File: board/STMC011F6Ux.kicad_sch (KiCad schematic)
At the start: 10 parts, among them J5 STDC14, SW1 SW_Push, U1 STM32C011F6Ux, Y1 48MHz

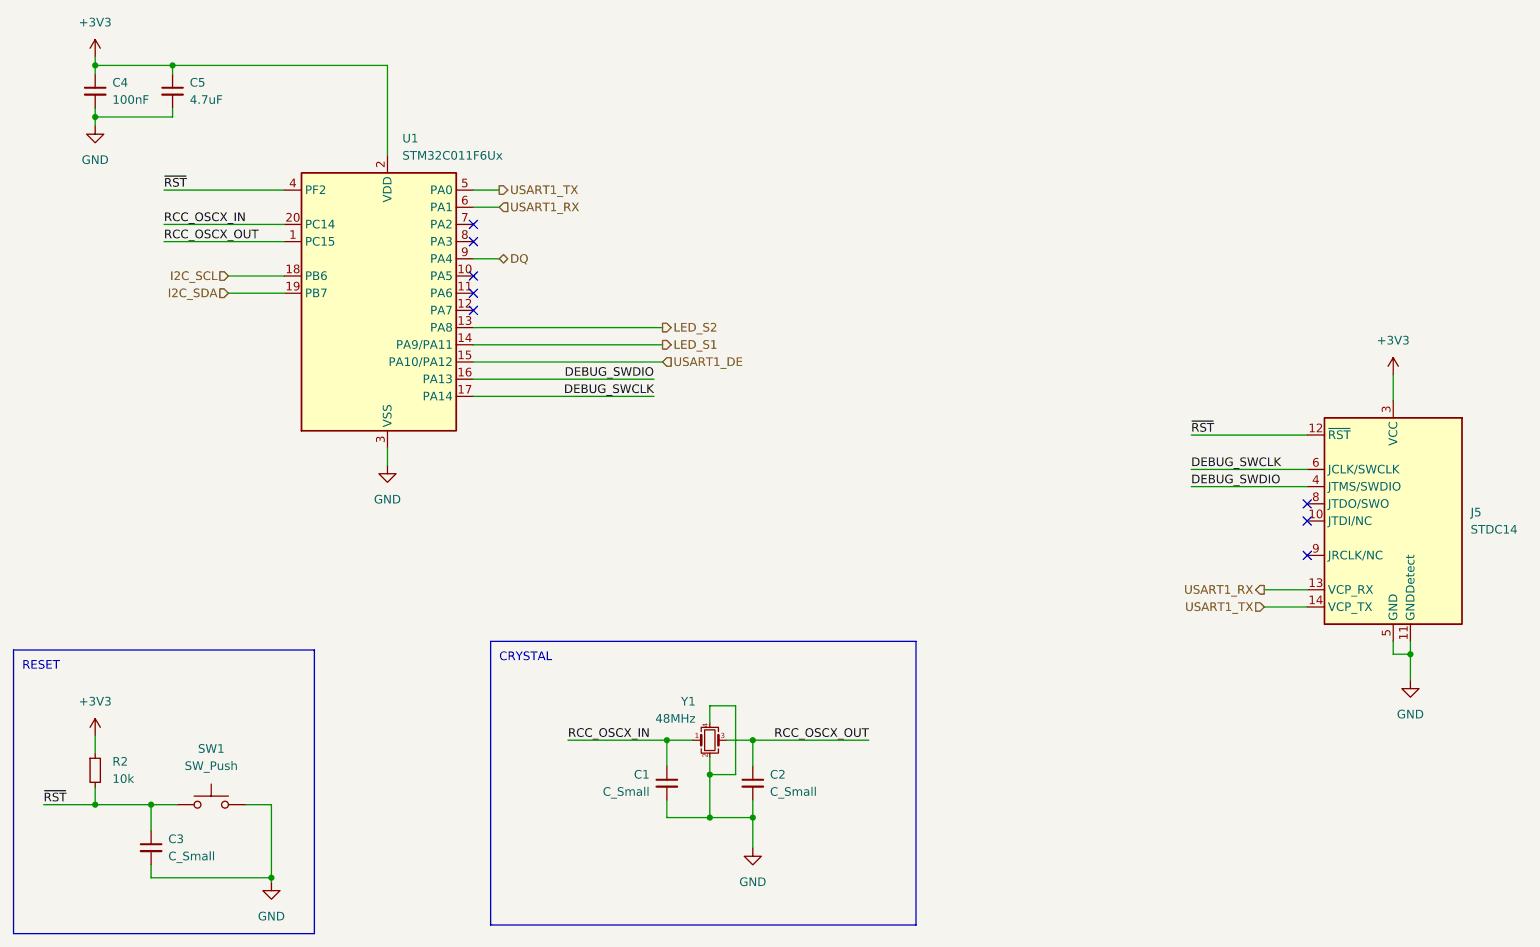
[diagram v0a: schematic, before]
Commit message: Final update
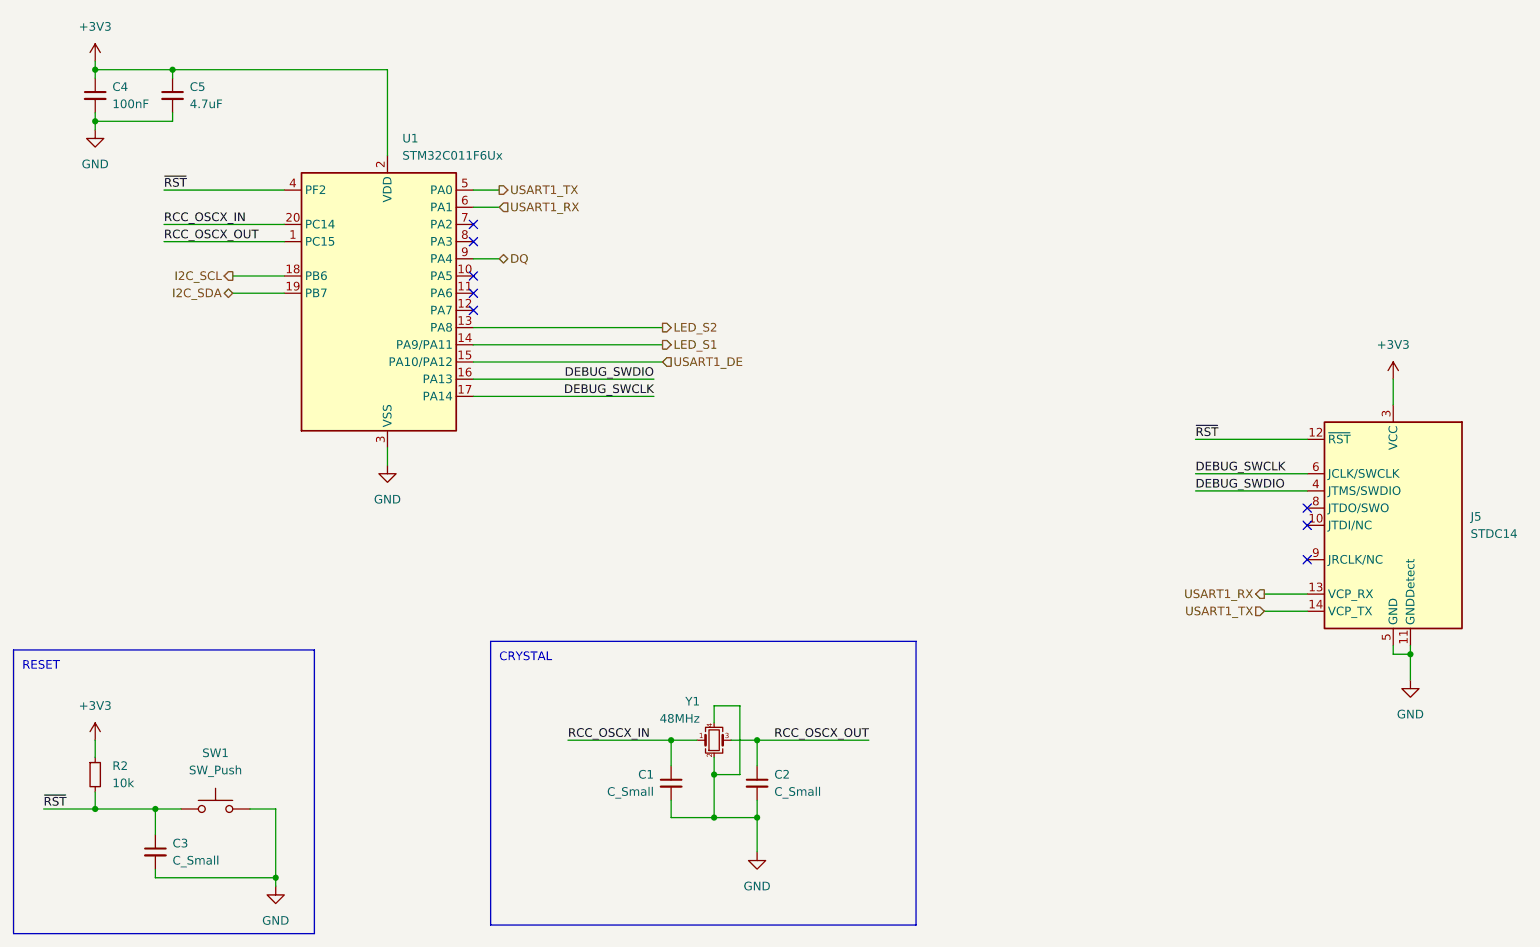
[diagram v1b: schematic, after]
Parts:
- SW1: footprint Connector_PinHeader_2.54mm:PinHeader_1x02_P2.54mm_Vertical -> Aliexpress:Push_Button_G71Y_3X6X3.5MM
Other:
- moved on the sheet: C1, C2, C3, C4, C5, J5, R2, SW1, Y1
